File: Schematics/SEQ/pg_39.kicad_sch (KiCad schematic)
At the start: 22 parts, among them U4001 F280, U4002 F280, U4003 F280, U4004 F280, U4005 F280, U4006 F280, U4007 F280, U4008 F280, U4009 F240, U4010 F521, U4011 F51, U4012 F37

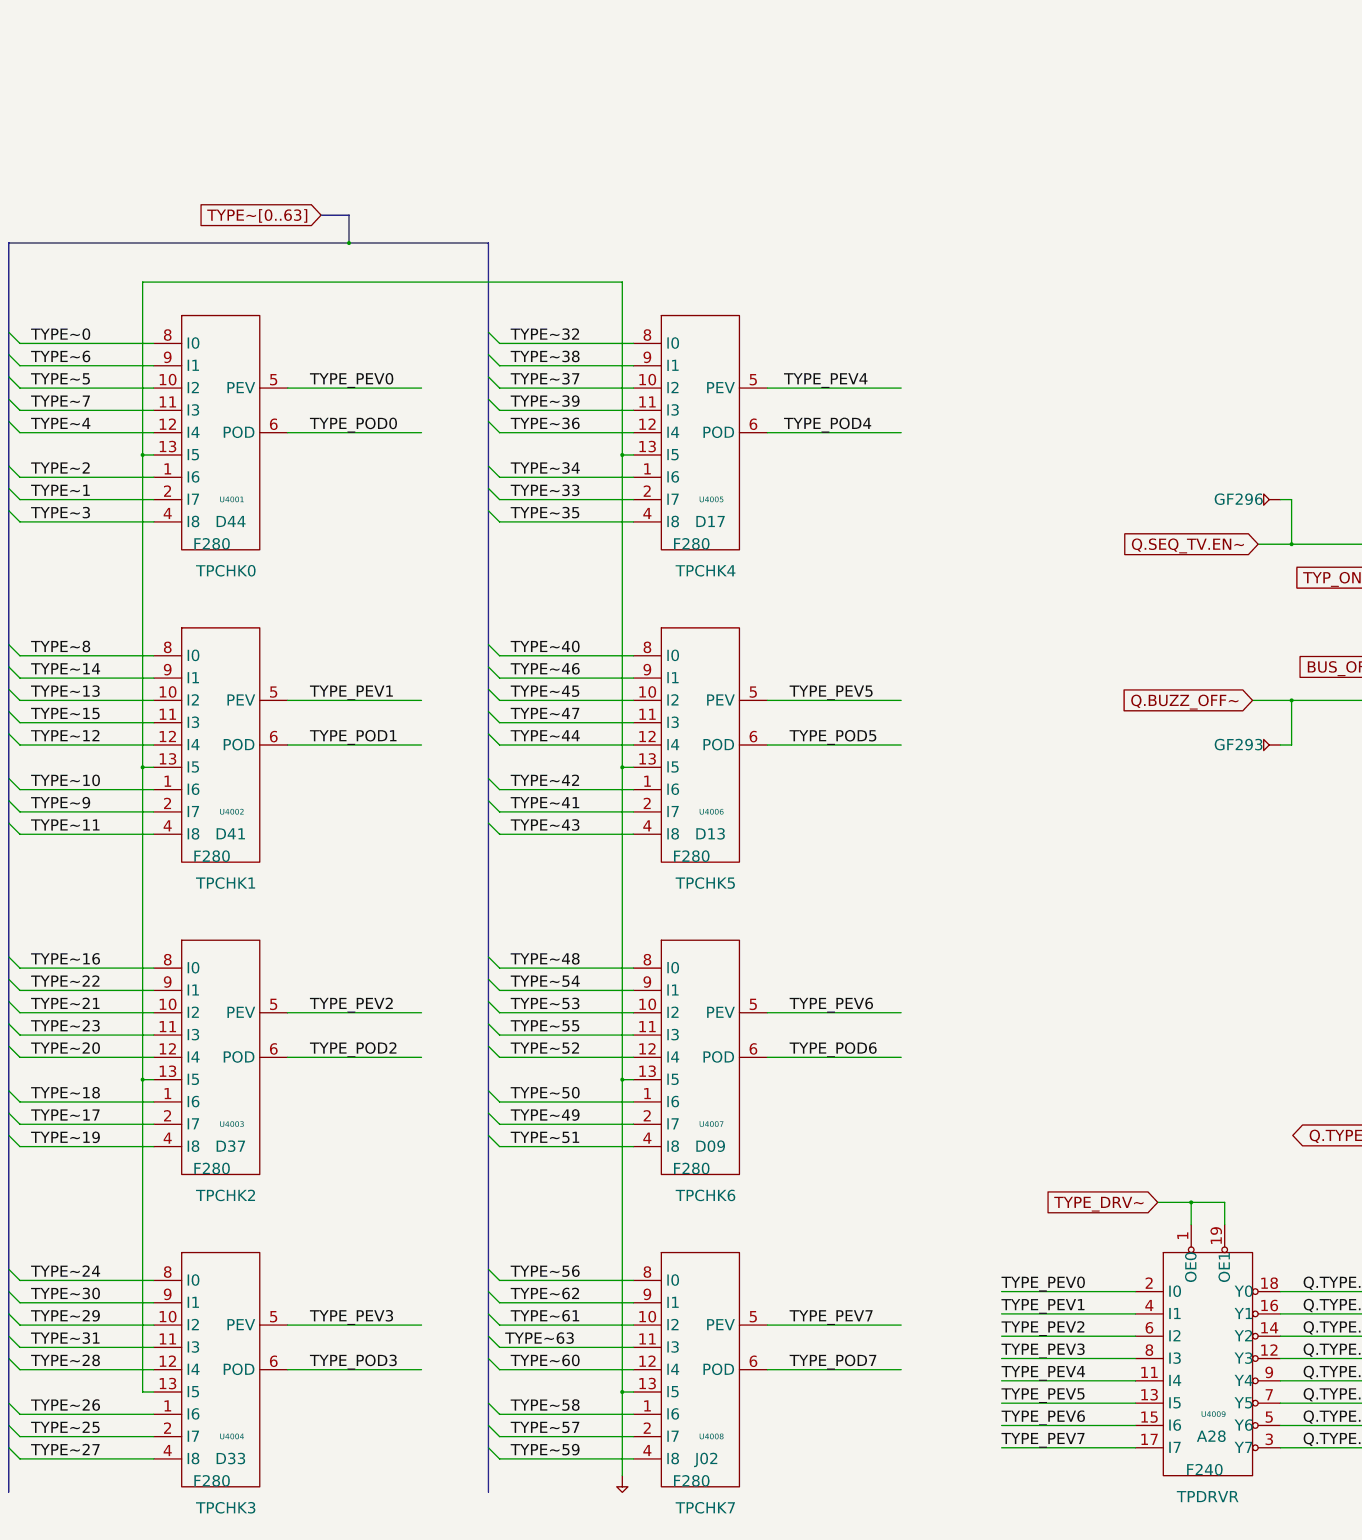
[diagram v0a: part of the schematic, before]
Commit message: Much work on SEQ
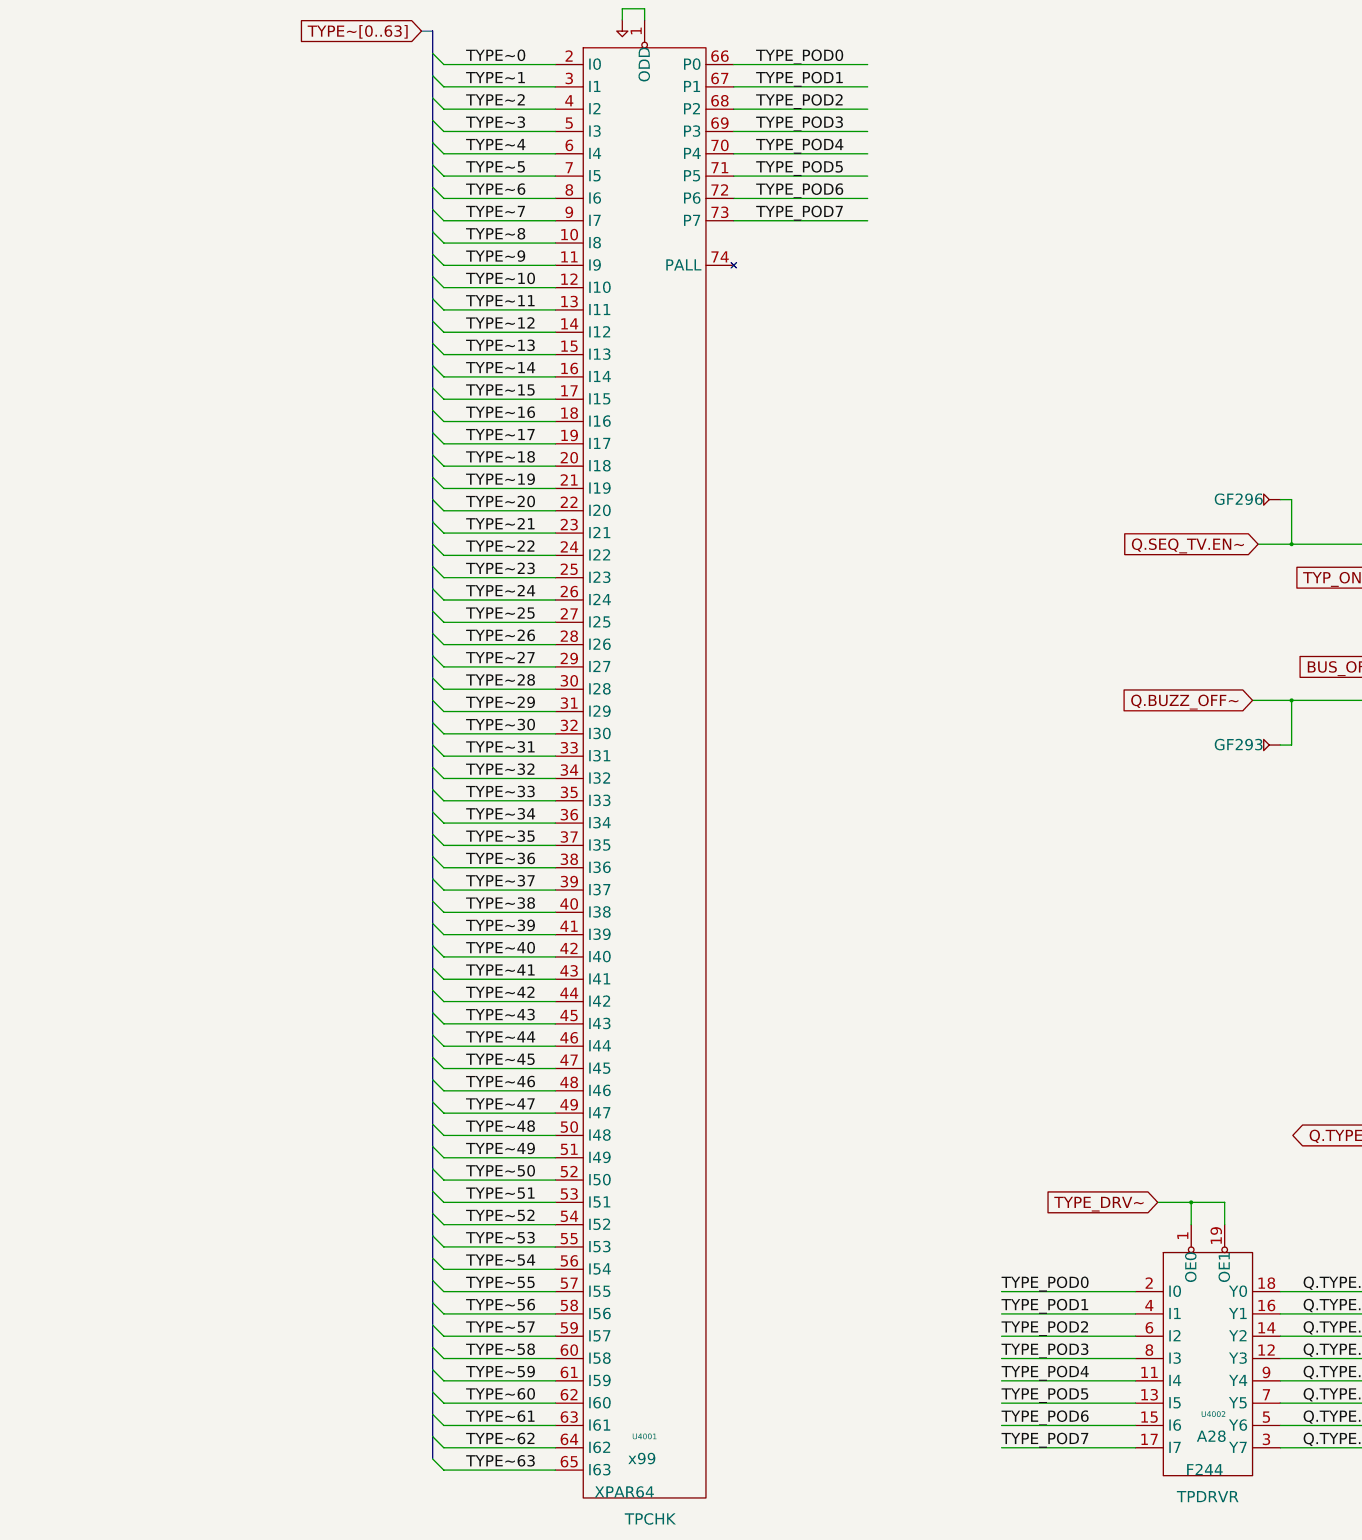
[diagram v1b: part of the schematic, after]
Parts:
- removed U4003, U4004, U4005, U4006, U4007, U4008: F280, symbol r1000:F280
- removed U4009: F240, symbol r1000:F240
- U4001: value F280 -> XPAR64; symbol r1000:F280 -> r1000:XPAR64; Location D44 -> x99; Name TPCHK0 -> TPCHK
- U4002: value F280 -> F244; symbol r1000:F280 -> r1000:F244; Location D41 -> A28; Name TPCHK1 -> TPDRVR
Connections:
- net TYPE_PEV0 is gone; now on net TYPE~3: U4001.5 (I3)
- net TYPE_PEV1 is gone; now on net Q.TYPE.P6: U4002.5 (Y6)
- net PD: now also U4001.1 (ODD); no longer U4001.13 (I5), U4002.13 (I5)
- net Q.TYPE.P0: now also U4002.18 (Y0)
- net Q.TYPE.P1: now also U4002.16 (Y1)
- net Q.TYPE.P2: now also U4002.14 (Y2)
- net Q.TYPE.P3: now also U4002.12 (Y3)
- net Q.TYPE.P4: now also U4002.9 (Y4)
- net Q.TYPE.P5: now also U4002.7 (Y5)
- net Q.TYPE.P7: now also U4002.3 (Y7)
- net TYPE_DRV~: now also U4002.1 (OE0), U4002.19 (OE1)
- net TYPE_POD0: now also U4001.66 (P0), U4002.2 (I0); no longer U4001.6 (POD)
- net TYPE_POD1: now also U4001.67 (P1), U4002.4 (I1); no longer U4002.6 (POD)
- net TYPE_POD2: now also U4001.68 (P2), U4002.6 (I2)
- net TYPE_POD3: now also U4001.69 (P3), U4002.8 (I3)
- net TYPE_POD4: now also U4001.70 (P4), U4002.11 (I4)
- net TYPE_POD5: now also U4001.71 (P5), U4002.13 (I5)
- net TYPE_POD6: now also U4001.72 (P6), U4002.15 (I6)
- net TYPE_POD7: now also U4001.73 (P7), U4002.17 (I7)
- net TYPE~0: now also U4001.2 (I0); no longer U4001.8 (I0)
- net TYPE~1: now also U4001.3 (I1); no longer U4001.2 (I7)
- net TYPE~10: now also U4001.12 (I10); no longer U4002.1 (I6)
- net TYPE~11: now also U4001.13 (I11); no longer U4002.4 (I8)
- net TYPE~12: now also U4001.14 (I12); no longer U4002.12 (I4)
- net TYPE~13: now also U4001.15 (I13); no longer U4002.10 (I2)
- net TYPE~14: now also U4001.16 (I14); no longer U4002.9 (I1)
- net TYPE~15: now also U4001.17 (I15); no longer U4002.11 (I3)
- net TYPE~16: now also U4001.18 (I16)
- net TYPE~17: now also U4001.19 (I17)
- net TYPE~18: now also U4001.20 (I18)
- net TYPE~19: now also U4001.21 (I19)
- net TYPE~2: now also U4001.4 (I2); no longer U4001.1 (I6)
- net TYPE~20: now also U4001.22 (I20)
- net TYPE~21: now also U4001.23 (I21)
- net TYPE~22: now also U4001.24 (I22)
- net TYPE~23: now also U4001.25 (I23)
- net TYPE~24: now also U4001.26 (I24)
- net TYPE~25: now also U4001.27 (I25)
- net TYPE~26: now also U4001.28 (I26)
- net TYPE~27: now also U4001.29 (I27)
- net TYPE~28: now also U4001.30 (I28)
- net TYPE~29: now also U4001.31 (I29)
- net TYPE~3: no longer U4001.4 (I8)
- net TYPE~30: now also U4001.32 (I30)
- net TYPE~31: now also U4001.33 (I31)
- net TYPE~32: now also U4001.34 (I32)
- net TYPE~33: now also U4001.35 (I33)
- net TYPE~34: now also U4001.36 (I34)
- net TYPE~35: now also U4001.37 (I35)
- net TYPE~36: now also U4001.38 (I36)
- net TYPE~37: now also U4001.39 (I37)
- net TYPE~38: now also U4001.40 (I38)
- net TYPE~39: now also U4001.41 (I39)
- net TYPE~4: now also U4001.6 (I4); no longer U4001.12 (I4)
- net TYPE~40: now also U4001.42 (I40)
- net TYPE~41: now also U4001.43 (I41)
- net TYPE~42: now also U4001.44 (I42)
- net TYPE~43: now also U4001.45 (I43)
- net TYPE~44: now also U4001.46 (I44)
- net TYPE~45: now also U4001.47 (I45)
- net TYPE~46: now also U4001.48 (I46)
- net TYPE~47: now also U4001.49 (I47)
- net TYPE~48: now also U4001.50 (I48)
- net TYPE~49: now also U4001.51 (I49)
- net TYPE~5: now also U4001.7 (I5); no longer U4001.10 (I2)
- net TYPE~50: now also U4001.52 (I50)
- net TYPE~51: now also U4001.53 (I51)
- net TYPE~52: now also U4001.54 (I52)
- net TYPE~53: now also U4001.55 (I53)
- net TYPE~54: now also U4001.56 (I54)
- net TYPE~55: now also U4001.57 (I55)
- net TYPE~56: now also U4001.58 (I56)
- net TYPE~57: now also U4001.59 (I57)
- net TYPE~58: now also U4001.60 (I58)
- net TYPE~59: now also U4001.61 (I59)
- net TYPE~6: now also U4001.8 (I6); no longer U4001.9 (I1)
- net TYPE~60: now also U4001.62 (I60)
- net TYPE~61: now also U4001.63 (I61)
- net TYPE~62: now also U4001.64 (I62)
- net TYPE~63: now also U4001.65 (I63)
- net TYPE~7: now also U4001.9 (I7); no longer U4001.11 (I3)
- net TYPE~8: now also U4001.10 (I8); no longer U4002.8 (I0)
- net TYPE~9: now also U4001.11 (I9); no longer U4002.2 (I7)
- no-connect marks 0 -> 1
